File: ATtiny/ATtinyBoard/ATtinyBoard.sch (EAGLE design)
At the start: 4 parts, among them IC1 TINY13-20SSU

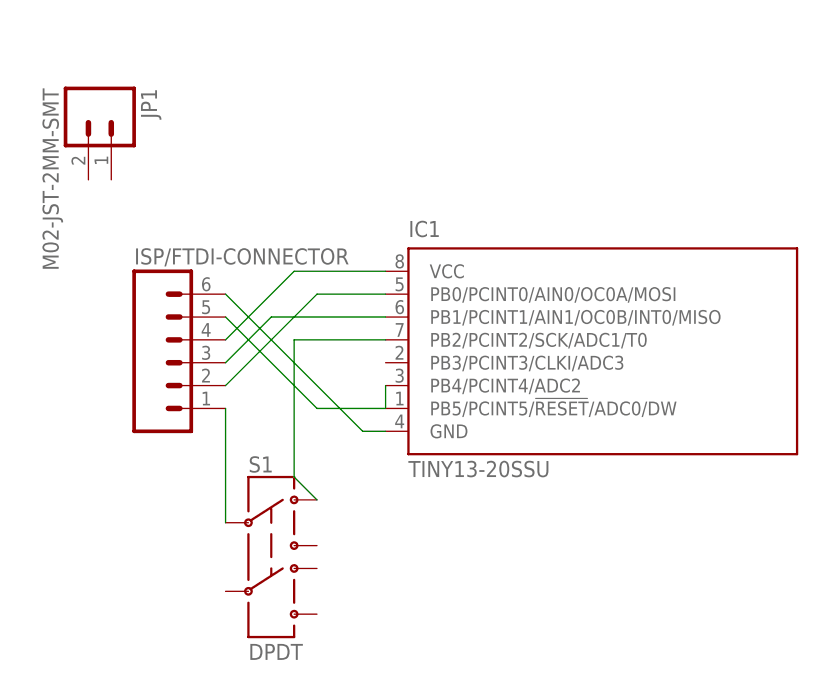
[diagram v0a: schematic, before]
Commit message: flex pcb stuff
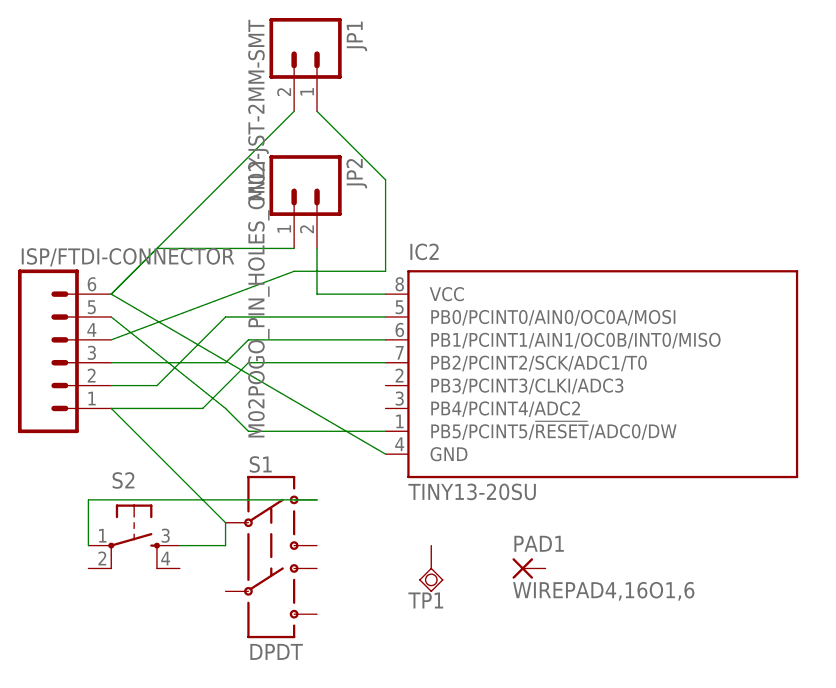
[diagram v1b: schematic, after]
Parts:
- removed IC1: TINY13-20SSU, atmel:TINY13-20SSU
- added IC2: TINY13-20SU, atmel:TINY13-20SU
- added JP2: M02POGO_PIN_HOLES_ONLY, SparkFun-Connectors:M02POGO_PIN_HOLES_ONLY
- added PAD1: WIREPAD4,16O1,6, wirepad:WIREPAD4,16O1,6
- added S2: (no value), SparkFun-Electromechanical:TAC_SWITCHSMD
- added TP1: TPSQTP20R, testpad:TPSQTP20R
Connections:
- removed net N$7: IC1.PB4/PCINT4/ADC2
- net N$1: now also IC2.PB0/PCINT0/AIN0/OC0A/MOSI, ISP/FTDI-CONNECTOR.2; no longer IC1.VCC, ISP/FTDI-CONNECTOR.4
- net N$2: now also IC2.GND, JP1.1, JP2.1; no longer IC1.GND
- net N$3: now also IC2.PB5/PCINT5/!RESET!/ADC0/DW; no longer IC1.PB5/PCINT5/!RESET!/ADC0/DW
- net N$4: now also IC2.PB1/PCINT1/AIN1/OC0B/INT0/MISO; no longer IC1.PB1/PCINT1/AIN1/OC0B/INT0/MISO
- net N$5: now also IC2.PB2/PCINT2/SCK/ADC1/T0, S2.3
- net N$6: now also IC2.VCC, ISP/FTDI-CONNECTOR.4, JP1.2, JP2.2; no longer IC1.PB0/PCINT0/AIN0/OC0A/MOSI, ISP/FTDI-CONNECTOR.2
- net N$8: now also S2.1; no longer IC1.PB2/PCINT2/SCK/ADC1/T0
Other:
- moved on the sheet: ISP/FTDI-CONNECTOR, JP1
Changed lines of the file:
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@@
 </classes>
 <parts>
-<part name="IC1" library="atmel" deviceset="TINY13" device="SSU" technology="-20"/>
 <part name="S1" library="SparkFun-Electromechanical" deviceset="SWITCH-DPDT" device="AYZ0202" value="DPDT"/>
 <part name="ISP/FTDI-CONNECTOR" library="SparkFun-Connectors" deviceset="M06" device="SMD"/>
 <part name="JP1" library="SparkFun-Connectors" deviceset="M02" device="-JST-2MM-SMT"/>
+<part name="S2" library="SparkFun-Electromechanical" deviceset="TAC_SWITCH" device="SMD"/>
+<part name="TP1" library="testpad" deviceset="TPSQ" device="TP20R"/>
+<part name="PAD1" library="wirepad" deviceset="WIREPAD" device="4,16O1,6"/>
+<part name="IC2" library="atmel" deviceset="TINY13" device="SU" technology="-20"/>
+<part name="JP2" library="SparkFun-Connectors" deviceset="M02" device="POGO_PIN_HOLES_ONLY"/>
 </parts>
 <sheets>
@@
 </plain>
 <instances>
-<instance part="IC1" gate="G$1" x="71.12" y="78.74"/>
 <instance part="S1" gate="G$1" x="38.1" y="60.96"/>
-<instance part="ISP/FTDI-CONNECTOR" gate="G$1" x="27.94" y="81.28"/>
-<instance part="JP1" gate="G$1" x="17.78" y="109.22" rot="R270"/>
+<instance part="ISP/FTDI-CONNECTOR" gate="G$1" x="15.24" y="81.28"/>
+<instance part="JP1" gate="G$1" x="40.64" y="116.84" rot="R270"/>
+<instance part="S2" gate="S" x="22.86" y="60.96"/>
+<instance part="TP1" gate="G$1" x="55.88" y="58.42"/>
+<instance part="PAD1" gate="G$1" x="66.04" y="58.42"/>
+<instance part="IC2" gate="G$1" x="71.12" y="76.2"/>
+<instance part="JP2" gate="G$1" x="40.64" y="101.6" rot="R270"/>
 </instances>
 <busses>
 </busses>
 <nets>
-<net name="N$1" class="0">
-<segment>
-<pinref part="IC1" gate="G$1" pin="VCC"/>
-<pinref part="ISP/FTDI-CONNECTOR" gate="G$1" pin="4"/>
-<wire x1="50.8" y1="91.44" x2="40.64" y2="91.44" width="0.1524" layer="91"/>
-<wire x1="40.64" y1="91.44" x2="33.02" y2="83.82" width="0.1524" layer="91"/>
-</segment>
-</net>
 <net name="N$2" class="0">
 <segment>
-<pinref part="IC1" gate="G$1" pin="GND"/>
 <pinref part="ISP/FTDI-CONNECTOR" gate="G$1" pin="6"/>
-<wire x1="50.8" y1="73.66" x2="48.26" y2="73.66" width="0.1524" layer="91"/>
-<wire x1="48.26" y1="73.66" x2="33.02" y2="88.9" width="0.1524" layer="91"/>
+<wire x1="50.8" y1="71.12" x2="20.32" y2="88.9" width="0.1524" layer="91"/>
+<pinref part="JP1" gate="G$1" pin="1"/>
+<wire x1="40.64" y1="109.22" x2="20.32" y2="88.9" width="0.1524" layer="91"/>
+<pinref part="IC2" gate="G$1" pin="GND"/>
+<pinref part="JP2" gate="G$1" pin="1"/>
+<wire x1="40.64" y1="93.98" x2="25.4" y2="93.98" width="0.1524" layer="91"/>
+<wire x1="25.4" y1="93.98" x2="20.32" y2="88.9" width="0.1524" layer="91"/>
 </segment>
 </net>
 <net name="N$3" class="0">
 <segment>
-<pinref part="IC1" gate="G$1" pin="PB5/PCINT5/!RESET!/ADC0/DW"/>
 <pinref part="ISP/FTDI-CONNECTOR" gate="G$1" pin="5"/>
-<wire x1="50.8" y1="76.2" x2="43.18" y2="76.2" width="0.1524" layer="91"/>
-<wire x1="43.18" y1="76.2" x2="33.02" y2="86.36" width="0.1524" layer="91"/>
-</segment>
-</net>
-<net name="N$4" class="0">
-<segment>
-<pinref part="IC1" gate="G$1" pin="PB1/PCINT1/AIN1/OC0B/INT0/MISO"/>
-<wire x1="50.8" y1="86.36" x2="38.1" y2="86.36" width="0.1524" layer="91"/>
-<pinref part="ISP/FTDI-CONNECTOR" gate="G$1" pin="3"/>
-<wire x1="38.1" y1="86.36" x2="33.02" y2="81.28" width="0.1524" layer="91"/>
+<wire x1="33.02" y1="76.2" x2="20.32" y2="86.36" width="0.1524" layer="91"/>
+<wire x1="33.02" y1="76.2" x2="35.56" y2="73.66" width="0.1524" layer="91"/>
+<pinref part="IC2" gate="G$1" pin="PB5/PCINT5/!RESET!/ADC0/DW"/>
+<wire x1="35.56" y1="73.66" x2="50.8" y2="73.66" width="0.1524" layer="91"/>
 </segment>
 </net>
 <net name="N$6" class="0">
 <segment>
-<pinref part="IC1" gate="G$1" pin="PB0/PCINT0/AIN0/OC0A/MOSI"/>
 <wire x1="50.8" y1="88.9" x2="43.18" y2="88.9" width="0.1524" layer="91"/>
-<pinref part="ISP/FTDI-CONNECTOR" gate="G$1" pin="2"/>
-<wire x1="43.18" y1="88.9" x2="33.02" y2="78.74" width="0.1524" layer="91"/>
-</segment>
-</net>
-<net name="N$7" class="0">
-<segment>
-<pinref part="IC1" gate="G$1" pin="PB4/PCINT4/ADC2"/>
-<wire x1="50.8" y1="78.74" x2="50.8" y2="76.2" width="0.1524" layer="91"/>
+<pinref part="IC2" gate="G$1" pin="VCC"/>
+<pinref part="ISP/FTDI-CONNECTOR" gate="G$1" pin="4"/>
+<wire x1="50.8" y1="91.44" x2="43.18" y2="91.44" width="0.1524" layer="91"/>
+<wire x1="43.18" y1="91.44" x2="40.64" y2="91.44" width="0.1524" layer="91"/>
+<wire x1="40.64" y1="91.44" x2="20.32" y2="83.82" width="0.1524" layer="91"/>
+<pinref part="JP1" gate="G$1" pin="2"/>
+<wire x1="43.18" y1="109.22" x2="50.8" y2="101.6" width="0.1524" layer="91"/>
+<wire x1="50.8" y1="101.6" x2="50.8" y2="91.44" width="0.1524" layer="91"/>
+<wire x1="43.18" y1="88.9" x2="43.18" y2="91.44" width="0.1524" layer="91"/>
+<pinref part="JP2" gate="G$1" pin="2"/>
+<wire x1="43.18" y1="91.44" x2="43.18" y2="93.98" width="0.1524" layer="91"/>
 </segment>
 </net>
@@
 <pinref part="ISP/FTDI-CONNECTOR" gate="G$1" pin="1"/>
 <pinref part="S1" gate="G$1" pin="2"/>
-<wire x1="33.02" y1="76.2" x2="33.02" y2="63.5" width="0.1524" layer="91"/>
+<wire x1="20.32" y1="76.2" x2="33.02" y2="63.5" width="0.1524" layer="91"/>
+<pinref part="S2" gate="S" pin="3"/>
+<wire x1="27.94" y1="60.96" x2="33.02" y2="60.96" width="0.1524" layer="91"/>
+<wire x1="33.02" y1="60.96" x2="33.02" y2="63.5" width="0.1524" layer="91"/>
+<pinref part="IC2" gate="G$1" pin="PB2/PCINT2/SCK/ADC1/T0"/>
+<wire x1="50.8" y1="81.28" x2="35.56" y2="81.28" width="0.1524" layer="91"/>
+<wire x1="35.56" y1="81.28" x2="30.48" y2="76.2" width="0.1524" layer="91"/>
+<wire x1="30.48" y1="76.2" x2="20.32" y2="76.2" width="0.1524" layer="91"/>
 </segment>
 </net>
 <net name="N$8" class="0">
 <segment>
-<pinref part="IC1" gate="G$1" pin="PB2/PCINT2/SCK/ADC1/T0"/>
-<wire x1="50.8" y1="83.82" x2="40.64" y2="83.82" width="0.1524" layer="91"/>
 <pinref part="S1" gate="G$1" pin="1"/>
-<wire x1="40.64" y1="83.82" x2="40.64" y2="68.58" width="0.1524" layer="91"/>
-<wire x1="40.64" y1="68.58" x2="43.18" y2="66.04" width="0.1524" layer="91"/>
+<pinref part="S2" gate="S" pin="1"/>
+<wire x1="43.18" y1="66.04" x2="17.78" y2="66.04" width="0.1524" layer="91"/>
+<wire x1="17.78" y1="66.04" x2="17.78" y2="60.96" width="0.1524" layer="91"/>
 </segment>
 </net>
+<net name="N$1" class="0">
+<segment>
+<pinref part="IC2" gate="G$1" pin="PB0/PCINT0/AIN0/OC0A/MOSI"/>
+<wire x1="50.8" y1="86.36" x2="33.02" y2="86.36" width="0.1524" layer="91"/>
+<wire x1="33.02" y1="86.36" x2="25.4" y2="78.74" width="0.1524" layer="91"/>
+<pinref part="ISP/FTDI-CONNECTOR" gate="G$1" pin="2"/>
+<wire x1="25.4" y1="78.74" x2="20.32" y2="78.74" width="0.1524" layer="91"/>
+</segment>
+</net>
+<net name="N$4" class="0">
+<segment>
+<pinref part="IC2" gate="G$1" pin="PB1/PCINT1/AIN1/OC0B/INT0/MISO"/>
+<wire x1="50.8" y1="83.82" x2="35.56" y2="83.82" width="0.1524" layer="91"/>
+<wire x1="35.56" y1="83.82" x2="33.02" y2="81.28" width="0.1524" layer="91"/>
+<pinref part="ISP/FTDI-CONNECTOR" gate="G$1" pin="3"/>
+<wire x1="33.02" y1="81.28" x2="20.32" y2="81.28" width="0.1524" layer="91"/>
+</segment>
+</net>
